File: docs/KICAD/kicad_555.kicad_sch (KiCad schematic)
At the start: 7 parts

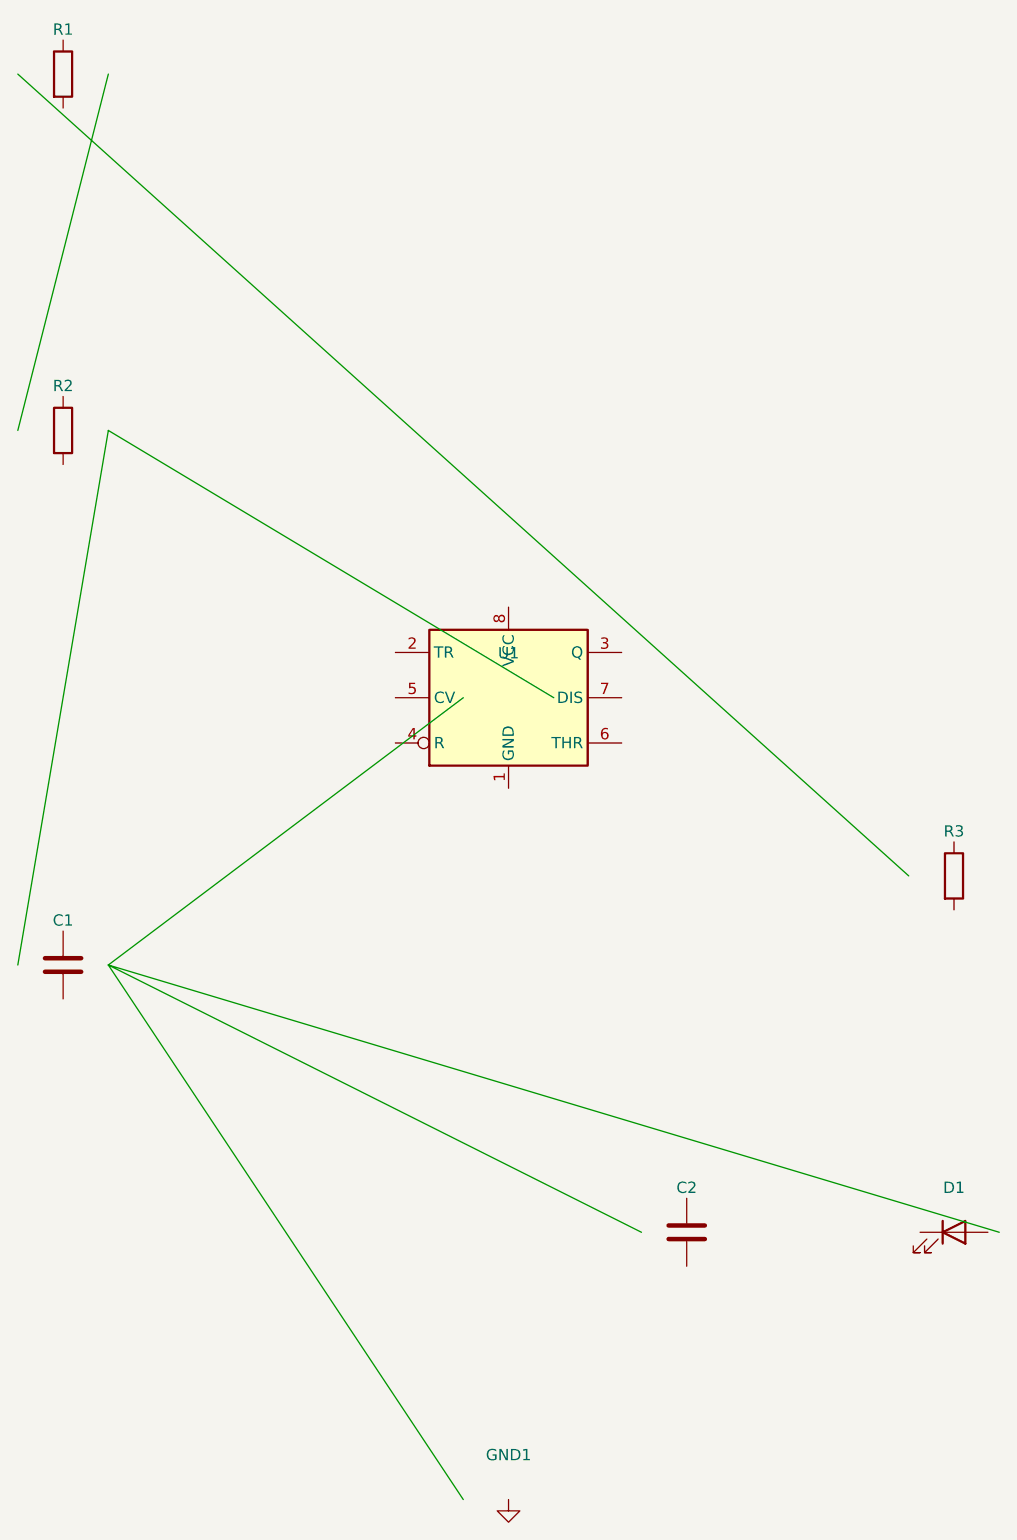
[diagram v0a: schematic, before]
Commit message: WIP: guardar cambios antes de pull
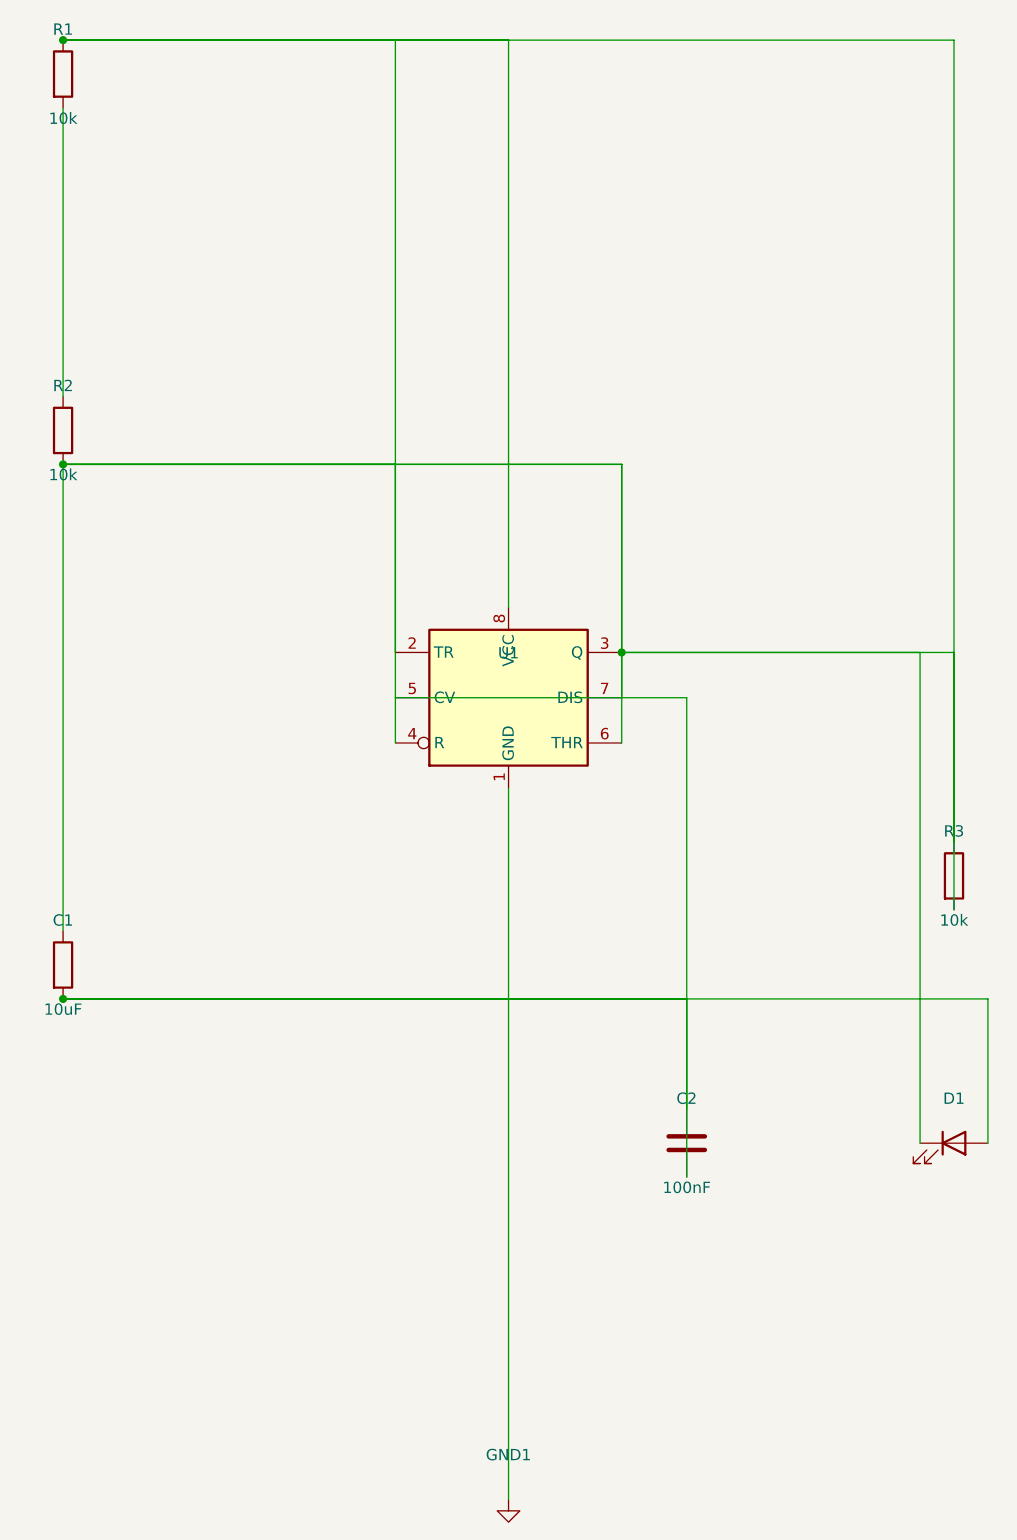
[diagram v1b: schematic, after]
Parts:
- removed C1: (no value), symbol Device:C
- added C1: 10uF, symbol Device:R
- C2: value (none) -> 100nF
- R1, R2, R3: value (none) -> 10k
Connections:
- net at R1.1: now also D1.1 (K), R2.2, R3.1, R3.2, U1.2 (TR), U1.3 (Q), U1.4 (R), U1.6 (THR), U1.7 (DIS), U1.8 (VCC), C1.1
- net at R1.2: now also R2.1
- net at D1.2 (A): now also C2.1, C2.2, U1.1 (GND), U1.5 (CV), C1.2
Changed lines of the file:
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@@
   (symbol (lib_id "Device:R") (at 50.0 30.0 0) (unit 1)
     (in_bom yes) (on_board yes) (dnp no)
-    (property "Reference" "R1" (at 50.0 25.0 0)
+    (property "Reference" "R1" (id 0) (at 50.0 25.0 0)
       (effects (font (size 1.27 1.27)))
     )
-    (property "Value" "" (at 50.0 35.0 0)
+    (property "Value" "10k" (id 1) (at 50.0 35.0 0)
       (effects (font (size 1.27 1.27)))
     )
@@
   (symbol (lib_id "Device:R") (at 50.0 70.0 0) (unit 1)
     (in_bom yes) (on_board yes) (dnp no)
-    (property "Reference" "R2" (at 50.0 65.0 0)
+    (property "Reference" "R2" (id 0) (at 50.0 65.0 0)
       (effects (font (size 1.27 1.27)))
     )
-    (property "Value" "" (at 50.0 75.0 0)
+    (property "Value" "10k" (id 1) (at 50.0 75.0 0)
       (effects (font (size 1.27 1.27)))
     )
@@
   (symbol (lib_id "Device:R") (at 150.0 120.0 0) (unit 1)
     (in_bom yes) (on_board yes) (dnp no)
-    (property "Reference" "R3" (at 150.0 115.0 0)
+    (property "Reference" "R3" (id 0) (at 150.0 115.0 0)
       (effects (font (size 1.27 1.27)))
     )
-    (property "Value" "" (at 150.0 125.0 0)
+    (property "Value" "10k" (id 1) (at 150.0 125.0 0)
       (effects (font (size 1.27 1.27)))
     )
   )
-  (symbol (lib_id "Device:C") (at 50.0 130.0 0) (unit 1)
+  (symbol (lib_id "Device:R") (at 50.0 130.0 0) (unit 1)
     (in_bom yes) (on_board yes) (dnp no)
-    (property "Reference" "C1" (at 50.0 125.0 0)
+    (property "Reference" "C1" (id 0) (at 50.0 125.0 0)
       (effects (font (size 1.27 1.27)))
     )
-    (property "Value" "" (at 50.0 135.0 0)
+    (property "Value" "10uF" (id 1) (at 50.0 135.0 0)
       (effects (font (size 1.27 1.27)))
     )
   )
-  (symbol (lib_id "Device:C") (at 120.0 160.0 0) (unit 1)
+  (symbol (lib_id "Device:C") (at 120.0 150.0 0) (unit 1)
     (in_bom yes) (on_board yes) (dnp no)
-    (property "Reference" "C2" (at 120.0 155.0 0)
+    (property "Reference" "C2" (id 0) (at 120.0 145.0 0)
       (effects (font (size 1.27 1.27)))
     )
-    (property "Value" "" (at 120.0 165.0 0)
+    (property "Value" "100nF" (id 1) (at 120.0 155.0 0)
       (effects (font (size 1.27 1.27)))
     )
   )
-  (symbol (lib_id "Device:LED") (at 150.0 160.0 0) (unit 1)
+  (symbol (lib_id "Device:LED") (at 150.0 150.0 0) (unit 1)
     (in_bom yes) (on_board yes) (dnp no)
-    (property "Reference" "D1" (at 150.0 155.0 0)
+    (property "Reference" "D1" (id 0) (at 150.0 145.0 0)
       (effects (font (size 1.27 1.27)))
     )
-    (property "Value" "" (at 150.0 165.0 0)
+    (property "Value" "" (id 1) (at 150.0 155.0 0)
       (effects (font (size 1.27 1.27)))
     )
@@
   (symbol (lib_id "Timer:NE555P") (at 100.0 100.0 0) (unit 1)
     (in_bom yes) (on_board yes) (dnp no)
-    (property "Reference" "U1" (at 100.0 95.0 0)
+    (property "Reference" "U1" (id 0) (at 100.0 95.0 0)
       (effects (font (size 1.27 1.27)))
     )
-    (property "Value" "" (at 100.0 105.0 0)
+    (property "Value" "" (id 1) (at 100.0 105.0 0)
       (effects (font (size 1.27 1.27)))
     )
@@
   (symbol (lib_id "power:GND") (at 100.0 190.0 0) (unit 1)
     (in_bom yes) (on_board yes) (dnp no)
-    (property "Reference" "GND1" (at 100.0 185.0 0)
+    (property "Reference" "GND1" (id 0) (at 100.0 185.0 0)
       (effects (font (size 1.27 1.27)))
     )
-    (property "Value" "" (at 100.0 195.0 0)
+    (property "Value" "" (id 1) (at 100.0 195.0 0)
       (effects (font (size 1.27 1.27)))
     )
   )
-  (wire (pts (xy 44.92 30.0) (xy 144.92 120.0))
+  (junction (at 50.0 26.19) (diameter 0) (color 0 0 0 0)
+  )
+  (wire (pts (xy 50.0 26.19) (xy 100.0 26.19))
     (stroke (width 0) (type default))
   )
-  (wire (pts (xy 55.08 130.0) (xy 94.92 100.0))
+  (wire (pts (xy 100.0 26.19) (xy 100.0 89.84))
     (stroke (width 0) (type default))
   )
-  (wire (pts (xy 55.08 130.0) (xy 114.92 160.0))
+  (wire (pts (xy 50.0 26.19) (xy 87.3 26.19))
     (stroke (width 0) (type default))
   )
-  (wire (pts (xy 55.08 130.0) (xy 155.08 160.0))
+  (wire (pts (xy 87.3 26.19) (xy 87.3 105.08))
     (stroke (width 0) (type default))
   )
-  (wire (pts (xy 55.08 130.0) (xy 94.92 190.0))
+  (wire (pts (xy 50.0 26.19) (xy 150.0 26.19))
     (stroke (width 0) (type default))
   )
-  (wire (pts (xy 55.08 30.0) (xy 44.92 70.0))
+  (wire (pts (xy 150.0 26.19) (xy 150.0 116.19))
     (stroke (width 0) (type default))
   )
-  (wire (pts (xy 55.08 70.0) (xy 44.92 130.0))
+  (junction (at 50.0 133.81) (diameter 0) (color 0 0 0 0)
+  )
+  (wire (pts (xy 50.0 133.81) (xy 100.0 133.81))
     (stroke (width 0) (type default))
   )
-  (wire (pts (xy 55.08 70.0) (xy 105.08 100.0))
+  (wire (pts (xy 100.0 133.81) (xy 100.0 110.16))
     (stroke (width 0) (type default))
   )
+  (wire (pts (xy 50.0 133.81) (xy 120.0 133.81))
+    (stroke (width 0) (type default))
+  )
+  (wire (pts (xy 120.0 133.81) (xy 120.0 153.81))
+    (stroke (width 0) (type default))
+  )
+  (wire (pts (xy 50.0 133.81) (xy 153.81 133.81))
+    (stroke (width 0) (type default))
+  )
+  (wire (pts (xy 153.81 133.81) (xy 153.81 150.0))
+    (stroke (width 0) (type default))
+  )
+  (wire (pts (xy 50.0 133.81) (xy 100.0 133.81))
+    (stroke (width 0) (type default))
+  )
+  (wire (pts (xy 100.0 133.81) (xy 100.0 190.0))
+    (stroke (width 0) (type default))
+  )
+  (wire (pts (xy 50.0 33.81) (xy 50.0 66.19))
+    (stroke (width 0) (type default))
+  )
+  (junction (at 50.0 73.81) (diameter 0) (color 0 0 0 0)
+  )
+  (wire (pts (xy 50.0 73.81) (xy 50.0 126.19))
+    (stroke (width 0) (type default))
+  )
+  (wire (pts (xy 50.0 73.81) (xy 87.3 73.81))
+    (stroke (width 0) (type default))
+  )
+  (wire (pts (xy 87.3 73.81) (xy 87.3 94.92))
+    (stroke (width 0) (type default))
+  )
+  (wire (pts (xy 50.0 73.81) (xy 112.7 73.81))
+    (stroke (width 0) (type default))
+  )
+  (wire (pts (xy 112.7 73.81) (xy 112.7 105.08))
+    (stroke (width 0) (type default))
+  )
+  (wire (pts (xy 50.0 73.81) (xy 112.7 73.81))
+    (stroke (width 0) (type default))
+  )
+  (wire (pts (xy 112.7 73.81) (xy 112.7 100.0))
+    (stroke (width 0) (type default))
+  )
+  (junction (at 112.7 94.92) (diameter 0) (color 0 0 0 0)
+  )
+  (wire (pts (xy 112.7 94.92) (xy 150.0 94.92))
+    (stroke (width 0) (type default))
+  )
+  (wire (pts (xy 150.0 94.92) (xy 150.0 123.81))
+    (stroke (width 0) (type default))
+  )
+  (wire (pts (xy 112.7 94.92) (xy 146.19 94.92))
+    (stroke (width 0) (type default))
+  )
+  (wire (pts (xy 146.19 94.92) (xy 146.19 150.0))
+    (stroke (width 0) (type default))
+  )
+  (wire (pts (xy 87.3 100.0) (xy 120.0 100.0))
+    (stroke (width 0) (type default))
+  )
+  (wire (pts (xy 120.0 100.0) (xy 120.0 146.19))
+    (stroke (width 0) (type default))
+  )
